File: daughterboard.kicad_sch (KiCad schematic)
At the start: 7 parts, among them J2 Conn_01x38, J3 Conn_01x38, J4 Conn_01x14, J5 Conn_02x11, J6 Conn_01x14, J7 Conn_01x38, J8 Conn_01x38

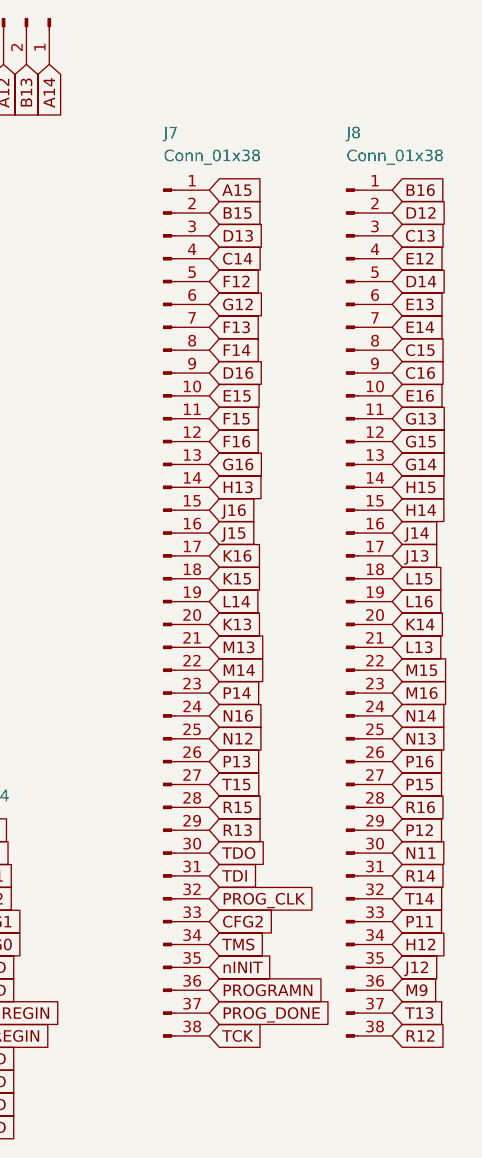
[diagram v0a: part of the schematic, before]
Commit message: Possibly finished PCB
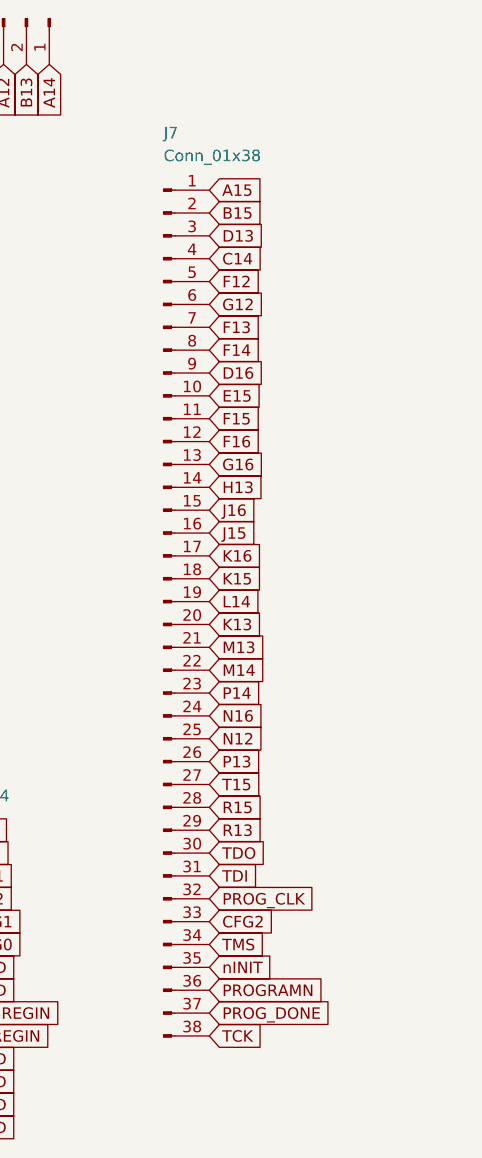
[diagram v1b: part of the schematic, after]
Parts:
- removed J8: Conn_01x38, Connector_PinHeader_1.27mm:PinHeader_1x38_P1.27mm_Vertical, symbol Connector:Conn_01x38_Pin
